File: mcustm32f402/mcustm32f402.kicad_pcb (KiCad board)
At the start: 2 copper layers, 76.2 x 50.8 mm, 37 parts, among them J2 STM32WORLD_CONNECTOR_1, J3 STM32WORLD_CONNECTOR_2, J4 STM32WORLD_BOARD, SW1 TS-1088R-02526, SW2 TS-1088R-02526, U1 AMS1117-3.3, U2 STM32F401RCTx, Y1 X_16MHZ

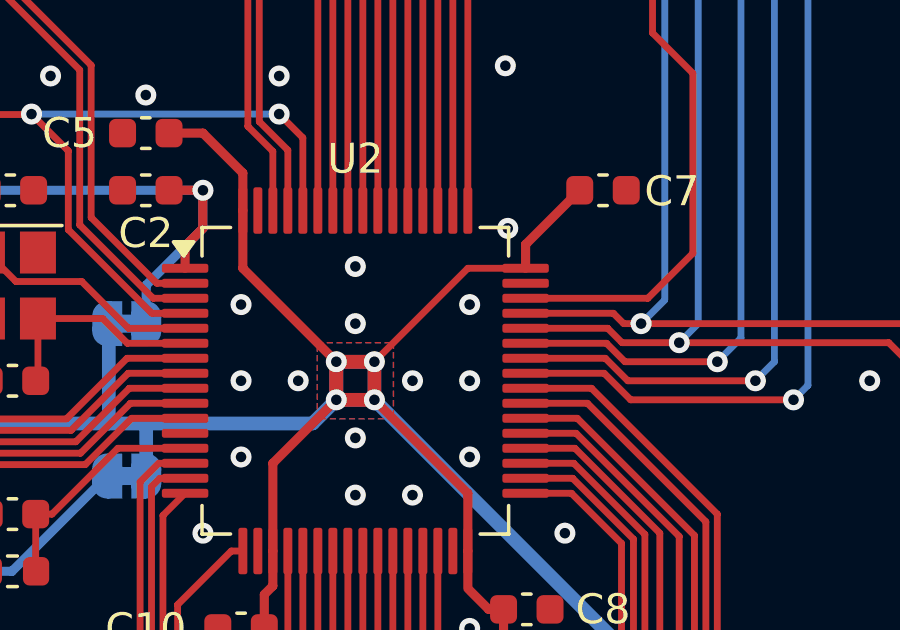
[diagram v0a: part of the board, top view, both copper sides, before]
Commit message: Hmmm
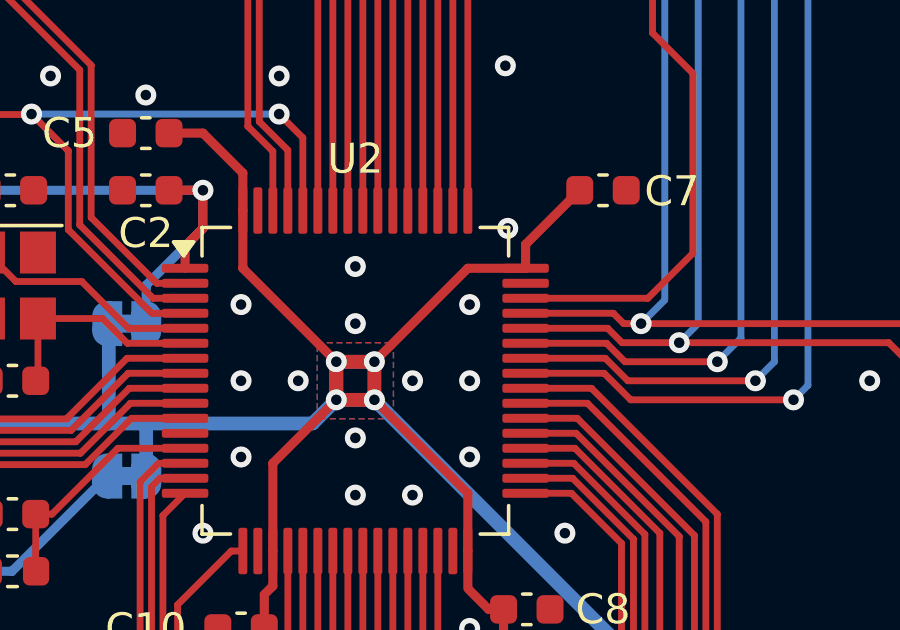
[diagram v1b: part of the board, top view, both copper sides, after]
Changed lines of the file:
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@@
 			)
 		)
-		(property "LCSC" "C72043"
+		(property "LCSC" "C19171301"
 			(at 0 0 0)
 			(layer "F.Fab")
@@
 			)
 		)
-		(property "LCSC" "C72041"
+		(property "LCSC" "C2288"
 			(at 0 0 0)
 			(layer "F.Fab")
@@
 			)
 		)
+		(property "LCSC" "C2915304"
+			(at 0 0 0)
+			(unlocked yes)
+			(layer "F.Fab")
+			(hide yes)
+			(effects
+				(font
+					(size 1 1)
+					(thickness 0.15)
+				)
+			)
+		)
 		(property ki_fp_filters "LQFP*10x10mm*P0.5mm*")
 		(sheetname "/")
@@
 	)
 	(segment
-		(start 158.075 97.85)
-		(end 156.15 97.85)
-		(width 0.2286)
-		(layer "F.Cu")
-		(net 1)
-	)
-	(segment
 		(start 149.365 108.725)
 		(end 149.365 109.855)
@@
 	)
 	(segment
+		(start 156.15 97.85)
+		(end 153.035 100.965)
+		(width 0.3048)
+		(layer "F.Cu")
+		(net 1)
+	)
+	(segment
 		(start 149.65 108.44)
 		(end 149.365 108.725)
@@
 	)
 	(segment
-		(start 156.15 97.85)
-		(end 153.035 100.965)
+		(start 115.91 110.49)
+		(end 115.91 113.03)
 		(width 0.2286)
 		(layer "F.Cu")
@@
 	)
 	(segment
-		(start 115.91 110.49)
-		(end 115.91 113.03)
-		(width 0.2286)
+		(start 158.075 97.85)
+		(end 156.15 97.85)
+		(width 0.3048)
 		(layer "F.Cu")
 		(net 1)
@@
 		(drill 0.35)
 		(layers "F.Cu" "B.Cu")
+		(locked yes)
 		(net 1)
 	)
@@
 		(drill 0.35)
 		(layers "F.Cu" "B.Cu")
+		(locked yes)
 		(net 1)
 	)
@@
 		(drill 0.35)
 		(layers "F.Cu" "B.Cu")
+		(locked yes)
 		(net 1)
 	)
@@
 		(drill 0.35)
 		(layers "F.Cu" "B.Cu")
+		(locked yes)
 		(net 1)
 	)
@@
 		(drill 0.35)
 		(layers "F.Cu" "B.Cu")
+		(locked yes)
 		(net 2)
 	)
@@
 		(drill 0.35)
 		(layers "F.Cu" "B.Cu")
+		(locked yes)
 		(net 2)
 	)
@@
 		(drill 0.35)
 		(layers "F.Cu" "B.Cu")
+		(locked yes)
 		(net 2)
 	)
@@
 		(drill 0.35)
 		(layers "F.Cu" "B.Cu")
+		(locked yes)
 		(net 2)
 	)
